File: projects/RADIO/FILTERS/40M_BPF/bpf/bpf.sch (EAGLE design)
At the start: 15 parts

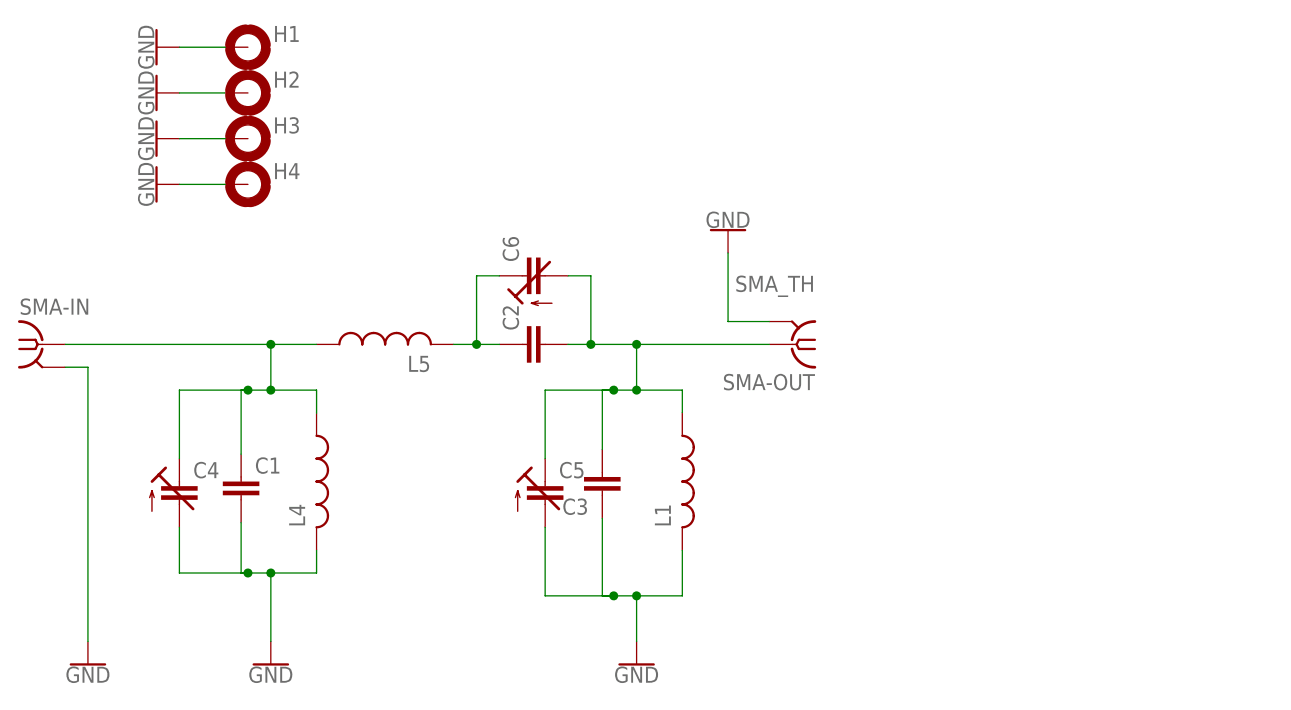
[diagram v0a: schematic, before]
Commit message: update
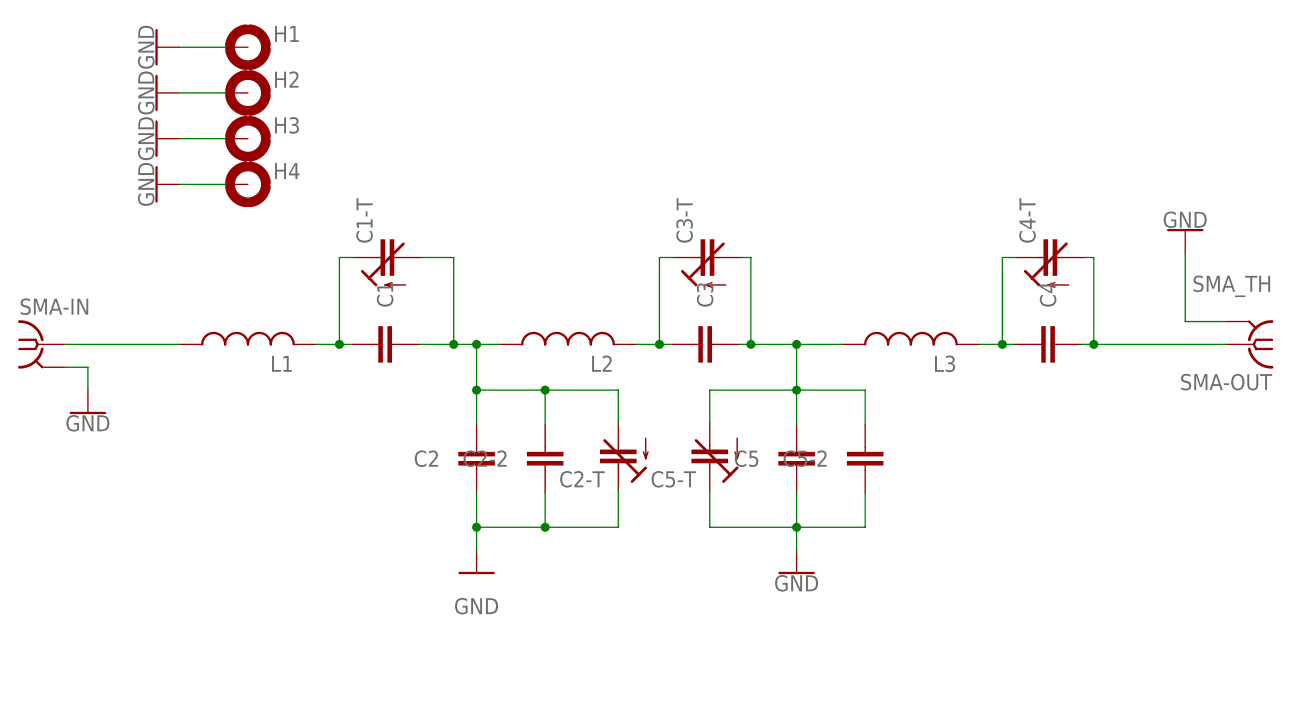
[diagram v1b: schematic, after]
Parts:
- removed C6: (no value), mylib:C_TRIM_TH
- removed L4: (no value), mylib:L_0805_PTH
- removed L5: (no value), mylib:L_WIRE_16MM
- added C1-T, C2-T, C3-T, C4-T, C5-T: (no value), mylib:C_TRIM_TH
- added C2-2, C5-2: (no value), mylib:C_0805_PTH
- added L2, L3: (no value), mylib:L_0805_PTH
- C4, C5: device mylib:C_TRIM_TH -> mylib:C_0805_PTH
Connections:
- removed net DIV: C2.1, C6.E, L5.2
- removed net IN: C1.1, C4.E, L4.1, L5.1, SMA-IN.1
- removed net OUT: C2.2, C3.2, C5.E, C6.A, L1.1, SMA-OUT.1
- new net N$1: L1.1, SMA-IN.1
- new net N$2: C1-T.E, C1.1, L1.2
- new net N$3: C1-T.A, C1.2, C2-2.2, C2-T.A, C2.2, L2.1
- new net N$4: C3-T.E, C3.1, L2.2
- new net N$5: C3-T.A, C3.2, C5-2.2, C5-T.A, C5.2, L3.1
- new net N$6: C4-T.E, C4.1, L3.2
- new net N$7: C4-T.A, C4.2, SMA-OUT.1
- net GND: now also C2-2.1, C2-T.E, C2.1, C5-2.1, C5-T.E, C5.1; no longer C1.2, C3.1, C4.A, C5.A, L1.2, L4.2
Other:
- moved on the sheet: C1, C2, C3, L1, SMA-OUT
